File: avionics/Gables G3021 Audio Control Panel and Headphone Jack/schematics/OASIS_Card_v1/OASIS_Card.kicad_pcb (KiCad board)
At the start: 2 copper layers, 106.4 x 46.2 mm, 55 parts, among them J1 Conn_02x08_Top_Bottom, J3 12v DC, J4 AudioJack3_Ground_Switch, J7 Piggyback Master, J8 Piggyback Slave, J9 12v DC, U1 CD4051B, U3 LTC1044

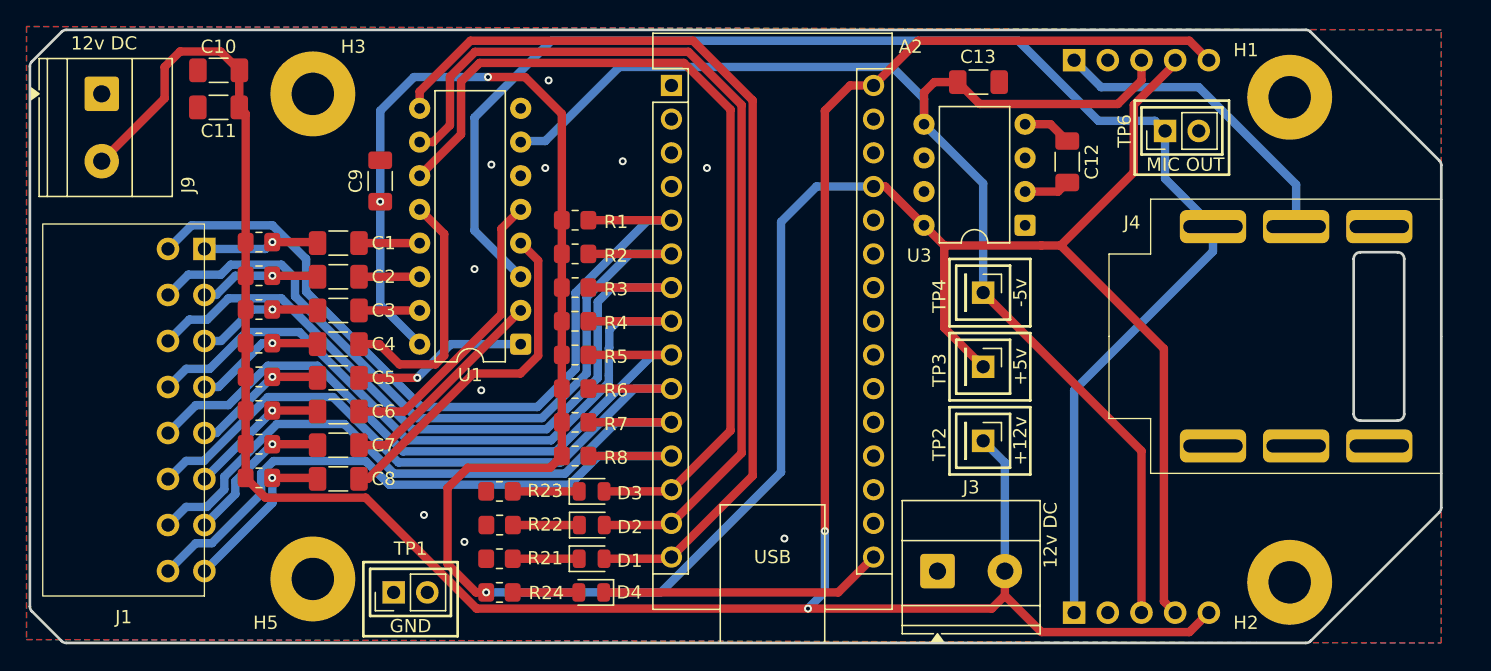
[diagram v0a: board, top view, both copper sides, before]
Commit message: more OASIS card stuff
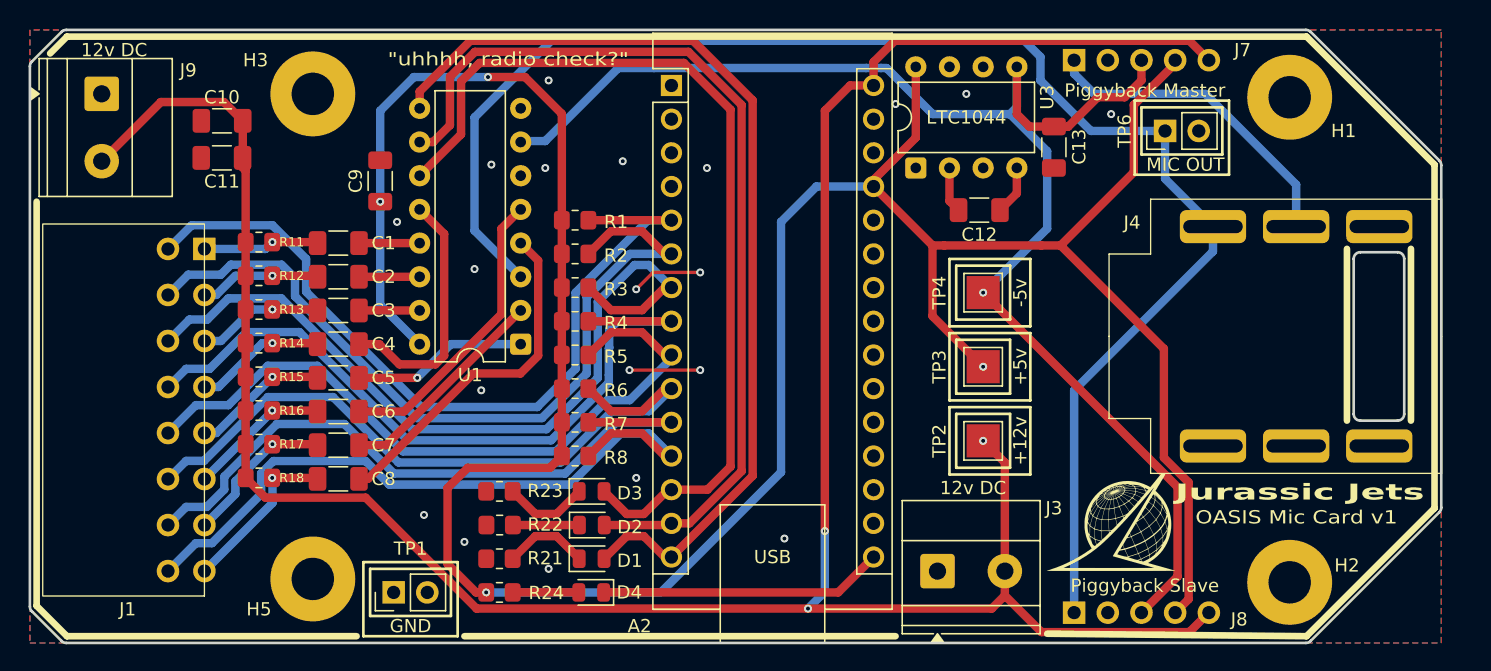
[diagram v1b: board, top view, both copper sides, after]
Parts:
- added G***: LOGO, LOGO, F.Cu at (184.7, 122.5)
- added G***: LOGO, LOGO, B.Cu at (156.6, 108.5)
- TP2, TP3, TP4: footprint Connector_PinHeader_2.54mm:PinHeader_1x01_P2.54mm_Vertical -> TestPoint:TestPoint_Pad_2.5x2.5mm
- moved U3 9.31 mm to (169.9, 95.8), turned to 90 degrees
- moved C12 7.57 mm to (174.7, 98.9), turned to 180 degrees
- moved C13 7.52 mm to (180.3, 94.2), turned to 90 degrees
- moved C10 3.82 mm to (117.6, 92.2)
- moved C11 3.82 mm to (117.6, 95.0)
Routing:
- net +5V: track 207.7 -> 219.3 mm, vias 3 -> 4
- net GND: track 0.02 -> 10.7 mm, vias 10 -> 20
- net -5V: track 101.4 -> 108.7 mm, vias 0 -> 1
- net +12V: track 207.7 -> 202.2 mm, vias 2 -> 3
- net Net-(A2-D10): track 66.0 -> 69.0 mm
- net Net-(A2-D4): track 56.9 -> 59.7 mm
- net Net-(A2-D9): track 49.7 -> 52.5 mm
- net Net-(A2-D6): track 51.5 -> 53.1 mm
- net Net-(D3-K): track 5.01 -> 6.43 mm
- net Net-(A2-D12): track 71.5 -> 72.9 mm
- net Net-(D1-K): track 5.01 -> 6.43 mm
- net Net-(A2-D3): track 58.8 -> 60.2 mm
- net Net-(A2-D7): track 50.6 -> 52.0 mm
- net Net-(J8-Pin_1): track 112.9 -> 113.9 mm
- net Net-(A2-D11): track 69.3 -> 70.1 mm
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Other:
- board text added: "Jurassic Jets"
- board text added: "OASIS Mic Card v1"
- board text added: "{dblquote}uhhhh, radio check?{dblquote}"
